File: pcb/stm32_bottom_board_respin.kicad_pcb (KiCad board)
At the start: 2 copper layers, 100 x 70 mm, 93 parts, among them J1 48V_SRC, J10 FCC_B2B, J11 SSR2_CTRL, J12 POWER, J13 PMS7003S_CONN, J14 MAINBOARD_CONN, J2 WS2812_CTRL, J3 FAN_CTRL, J4 SSR_OUTPUT, J5 PURFUME_CTRL, J6 Conn_01x14, J7 Conn_01x12, J8 Conn_01x15, J9 PCB_UART, Q1 2N3904(1AM), Q2 SS9013_J3, Q3 2N3904(1AM), Q4 2N3904(1AM), SW1 SW_Push, U1 74AHCT1G125, U2 OMRON-G3MB-202P, U3 STM32F103C8T6, U4 AMS1117-3.3, U5 SP3232EEN, U6 OMRON-G3MB-202P, U7 waveshare-swd-pinsocket, Y1 O8M, Y2 O_EPSON_32.768K

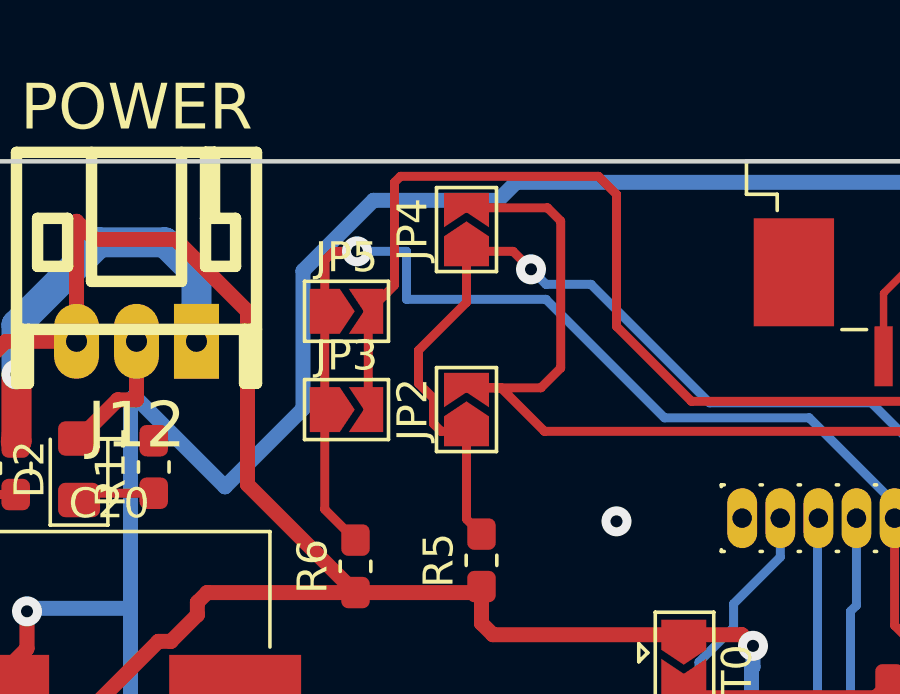
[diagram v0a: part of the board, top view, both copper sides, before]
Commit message: remove jumper,
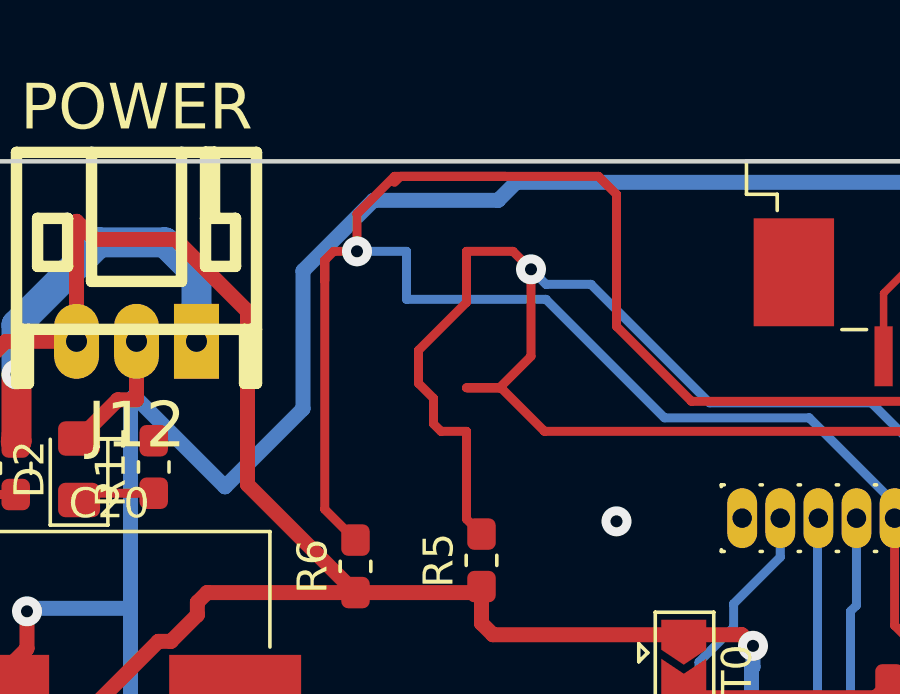
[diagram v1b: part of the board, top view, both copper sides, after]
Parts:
- removed JP2: SCL_EN, Jumper:SolderJumper-2_P1.3mm_Open_TrianglePad1.0x1.5mm
- removed JP3: SDA_EN, Jumper:SolderJumper-2_P1.3mm_Open_TrianglePad1.0x1.5mm
- removed JP4: TX_EN, Jumper:SolderJumper-2_P1.3mm_Open_TrianglePad1.0x1.5mm
- removed JP5: RX_EN, Jumper:SolderJumper-2_P1.3mm_Open_TrianglePad1.0x1.5mm
- R5, R6: value R472,0603 -> R472,0603,NC
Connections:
- J10 pad 6: Net-(J10-Pad6) -> B2B_UART_TX
- J10 pad 7: Net-(J10-Pad7) -> B2B_UART_RX
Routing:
- net Net-(J10-Pad7): track 32.4 -> 0.00 mm
- net B2B_UART_RX: track 51.7 -> 82.8 mm
- net Net-(J10-Pad6): track 30.2 -> 0.00 mm
- net B2B_UART_TX: track 45.6 -> 69.6 mm

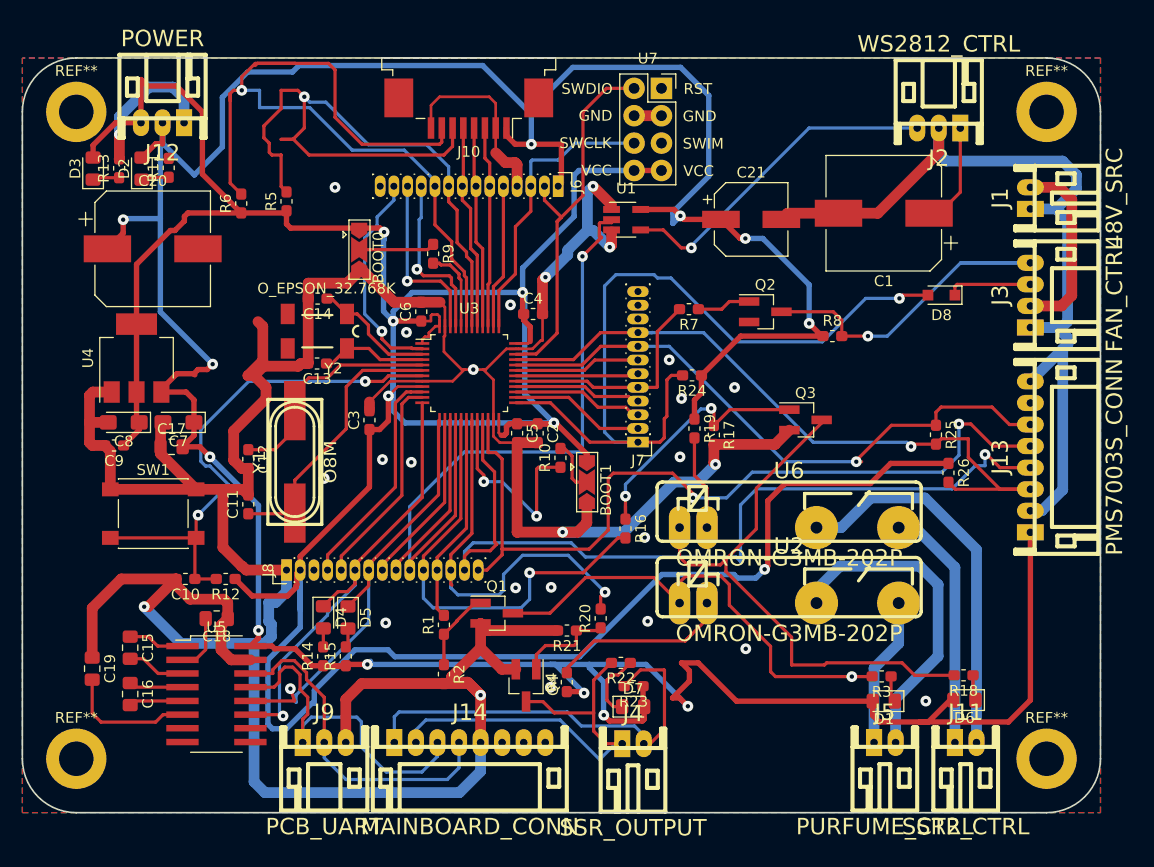
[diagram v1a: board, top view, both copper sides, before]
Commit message: update,
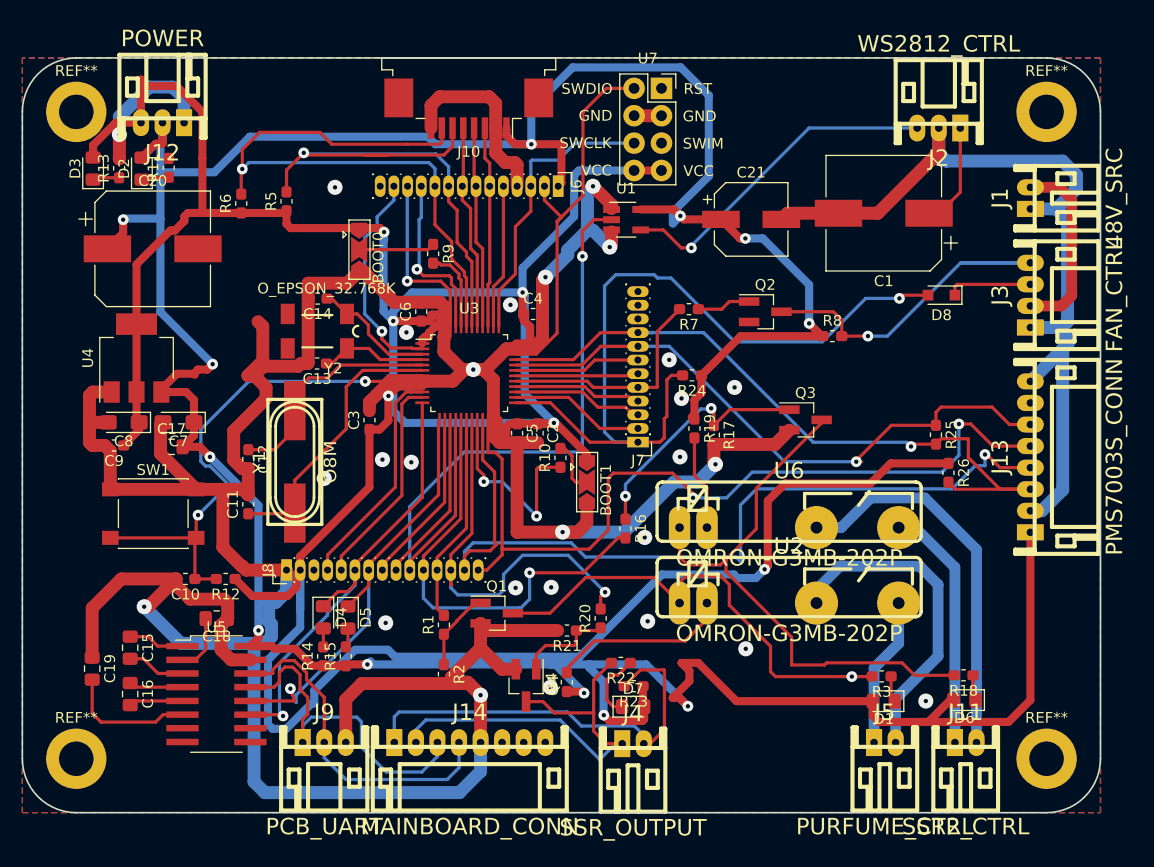
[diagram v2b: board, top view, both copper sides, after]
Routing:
- net B2B_UART_RX: track 82.8 -> 62.3 mm
- net B2B_UART_TX: track 69.6 -> 52.1 mm
- net +5V: track 333.2 -> 323.5 mm
- net +3V3: track 312.8 -> 311.3 mm
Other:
- net class GND: trace_width 1 -> 1.2; via_dia 1 -> 1.4
- net class HIGH_PWR: via_dia 1 -> 1.2
- net class PWR: trace_width 0.5 -> 0.75
